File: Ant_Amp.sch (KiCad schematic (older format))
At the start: 26 parts, among them J1 Conn_Coaxial, Q1 BF981

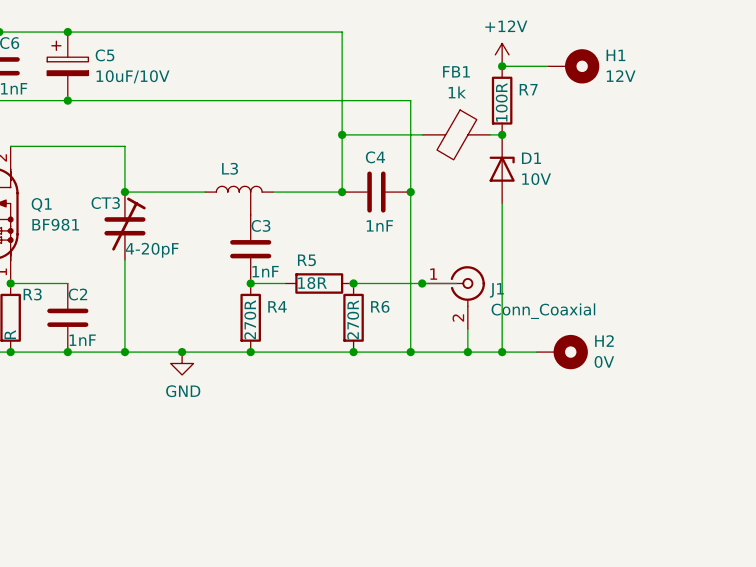
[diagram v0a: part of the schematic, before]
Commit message: 17-2-21_03
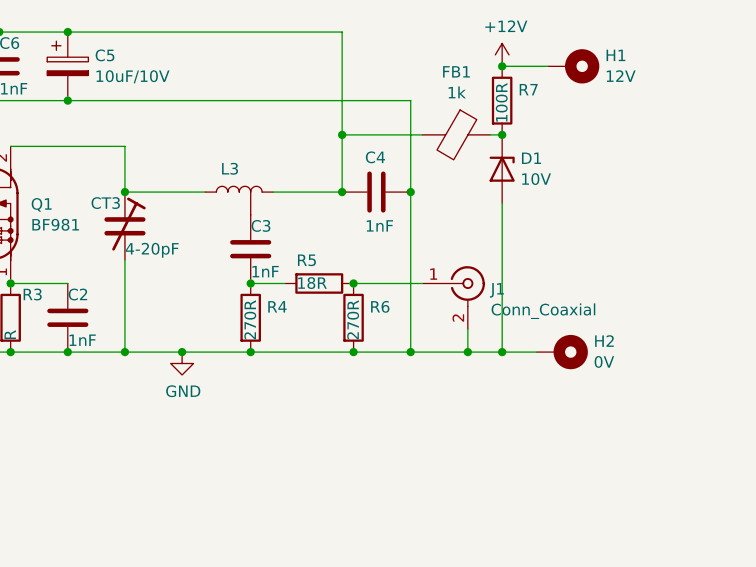
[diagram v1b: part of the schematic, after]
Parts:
- L1: footprint Inductor:L_6T_11mm_intdiam6.3mm_1mm_wire_tap1.5TL -> Inductor:L_6T_11mm_intdiam6.3mm_1mm_wire_tap4.5TR
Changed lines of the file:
@@
 F 0 "L1" H 2550 3350 50  0000 L CNN
 F 1 "L-Tap" H 2653 3105 50  0001 L CNN
-F 2 "Inductor:L_6T_11mm_intdiam6.3mm_1mm_wire_tap1.5TL" H 2600 3150 50  0001 C CNN
+F 2 "Inductor:L_6T_11mm_intdiam6.3mm_1mm_wire_tap4.5TR" H 2600 3150 50  0001 C CNN
 F 3 "~" H 2600 3150 50  0001 C CNN
 	1    2600 3150
@@
 $EndComp
 Wire Wire Line
-	5650 3000 5800 3000
-Wire Wire Line
-	5350 3000 5650 3000
-Connection ~ 5350 3000
-Connection ~ 5650 3000
-Wire Wire Line
 	5850 3200 5850 3300
 Connection ~ 5850 3300
@@
 	6150 3300 6000 3300
 Connection ~ 6000 3300
+Wire Wire Line
+	5650 3000 5350 3000
+Connection ~ 5350 3000
 $EndSCHEMATC

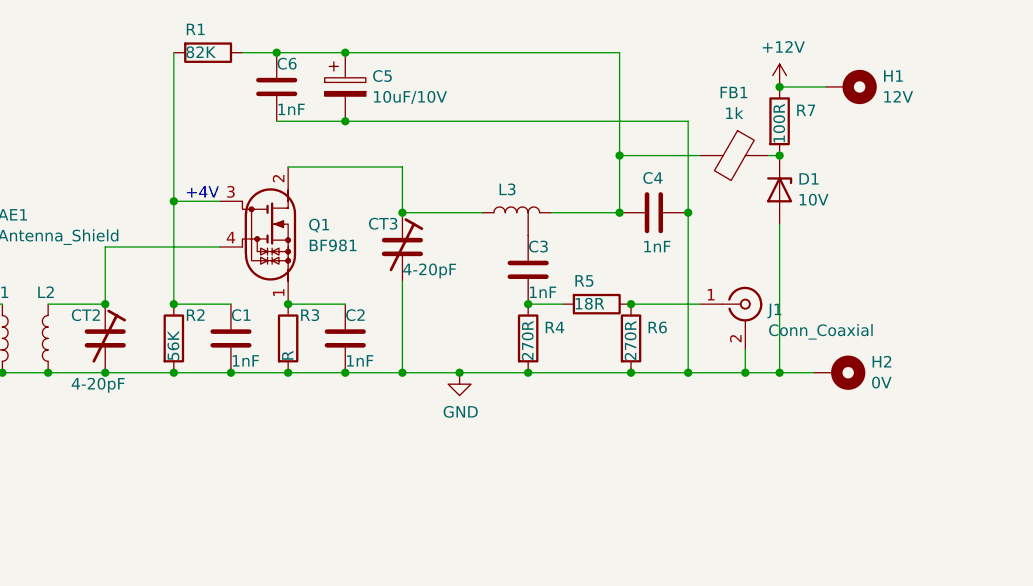
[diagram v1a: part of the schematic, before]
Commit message: Ver 1.0
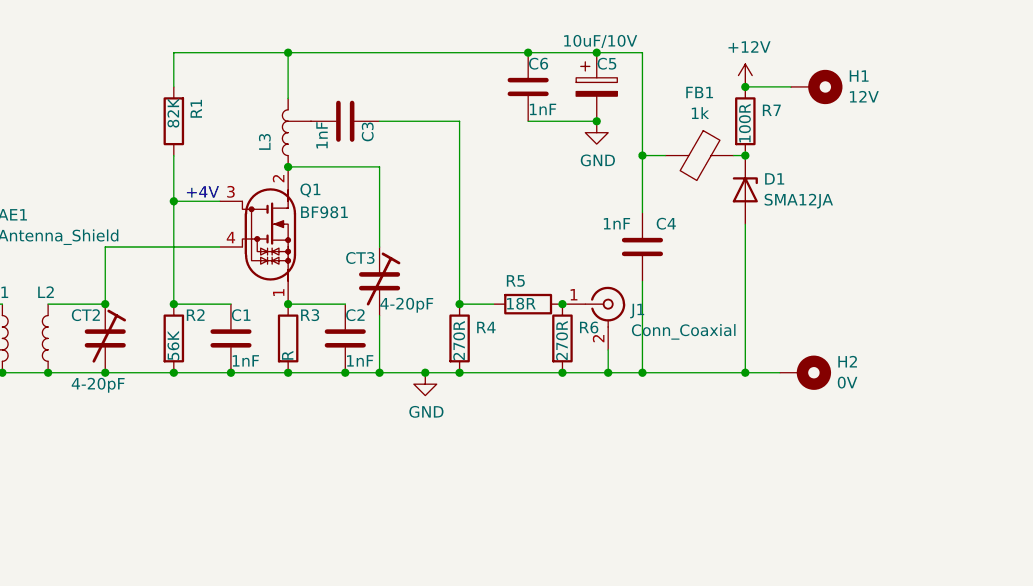
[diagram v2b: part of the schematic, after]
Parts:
- C1, C2, C3, C4, C6: footprint Capacitor_SMD:C_0603_1608Metric -> Capacitor_SMD:C_0402_1005Metric
- CT1, CT2, CT3: footprint Capacitor_SMD:C_Trimmer_Voltronics_JR -> Capacitor_SMD:C_Trimmer_Voltronics_JZ
- D1: value 10V -> SMA12JA
- R7: footprint Resistor_SMD:R_0603_1608Metric -> Resistor_SMD:R_2512_6332Metric
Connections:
- net at C4.2, C5.1, C6.1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: now also R1.2; no longer R1.1
- net at C1.1, Q1.3 (G2), R2.1: now also R1.1; no longer R1.2
- net at L3.3: now also C3.2; no longer C3.1
- net at R4.1, R5.2: now also C3.1; no longer C3.2
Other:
- moved on the sheet: C3, C4, C5, C6, CT3, D1, FB1, H1, H2, J1, L3, R1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
